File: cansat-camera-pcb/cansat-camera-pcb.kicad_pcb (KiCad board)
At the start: 8 copper layers, 50 x 50 mm, 69 parts, among them IC2 TLV74315PDBVR, J2 Micro_SD_Card_Det2, J3 Conn_01x05_Socket, J4 Conn_02x10_Odd_Even, J5 Conn_02x10_Odd_Even, J6 OV5640, SW2 SW_Push, U2 AP2112K-3.3, U3 W9825G6KH-6, U4 STM32H743ZITx, U6 TLV74328PDBVR, Y1 24MHz

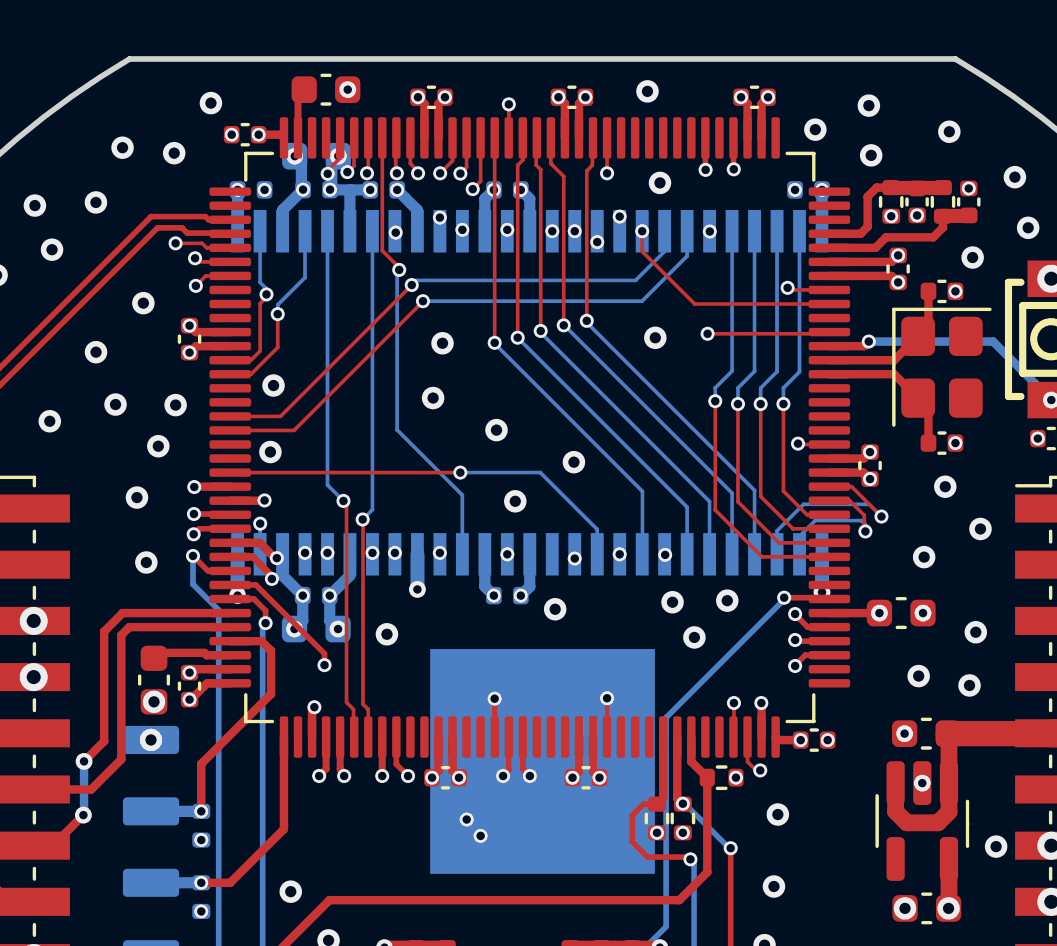
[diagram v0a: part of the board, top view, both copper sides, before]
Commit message: Routolás sdram
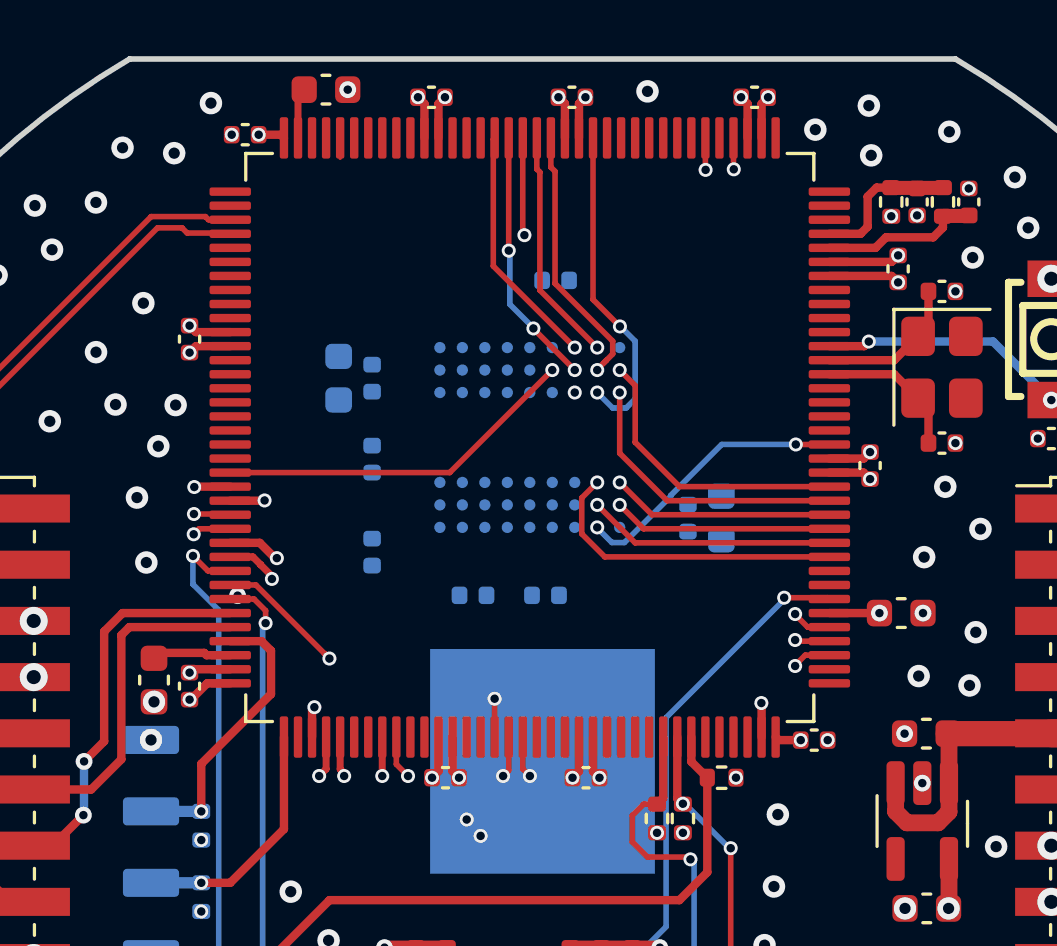
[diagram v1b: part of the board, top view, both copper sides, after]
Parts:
- removed U3: W9825G6KH-6, Package_SO:TSOP-II-54_22.2x10.16mm_P0.8mm
- added IC1: W9825G6JB-6I, Package_BGA:Alliance_TFBGA-54_8x8mm_Layout9x9_P0.8mm, B.Cu at (73.5, 116.1)
- moved C29 20.2 mm to (67.9, 120.2), turned to -90 degrees
- moved C32 16.5 mm to (71.5, 121.7), turned to 180 degrees
- moved C28 14.9 mm to (80.3, 119.0), turned to 90 degrees
- moved C30 13.5 mm to (79.1, 119.0), turned to 90 degrees
- moved C27 10.7 mm to (67.9, 116.9), turned to 90 degrees
- moved C33 7.94 mm to (66.7, 114.0), turned to 90 degrees
- moved C25 7.00 mm to (67.9, 114.0), turned to 90 degrees
- moved C26 6.91 mm to (74.4, 110.5), turned to 0 degrees
- moved C31 1.36 mm to (74.0, 121.7)
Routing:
- net /FMC_NBL0: track 21.2 -> 0.00 mm, vias 2 -> 0
- net /FMC_BS1: track 19.7 -> 0.00 mm, vias 1 -> 0
- net /FMC_BS0: track 18.6 -> 0.00 mm, vias 1 -> 0
- net /FMC_D2: track 18.4 -> 0.03 mm, vias 1 -> 0
- net /FMC_D3: track 18.2 -> 0.00 mm, vias 1 -> 0
- net /FMC_SDNCAS: track 17.8 -> 0.00 mm, vias 2 -> 0
- net /FMC_D13: track 17.7 -> 0.00 mm, vias 2 -> 0
- net /FMC_D8: track 17.1 -> 0.03 mm, vias 2 -> 0
- net /FMC_D9: track 16.1 -> 0.00 mm, vias 1 -> 0
- net /FMC_D10: track 15.9 -> 0.00 mm, vias 2 -> 0
- net /FMC_D11: track 15.6 -> 0.01 mm, vias 2 -> 0
- net /FMC_D14: track 15.2 -> 0.00 mm, vias 2 -> 0
- net /FMC_D15: track 15.1 -> 0.00 mm, vias 2 -> 0
- net /FMC_D12: track 15.8 -> 0.72 mm, vias 2 -> 0
- net GND: track 36.0 -> 21.5 mm, vias 170 -> 145
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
